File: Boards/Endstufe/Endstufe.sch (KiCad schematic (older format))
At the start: 55 parts, among them J1 HV In, J2 Relais, J3 Audio_In, J4 Übertrager, J5 Gegenkopplung, K1 G6E, P4 6V3_AC, P6 6V3_DC, P8 Bias, T1 KT88, T2 KT88, U1 ECC82, U2 ECC83

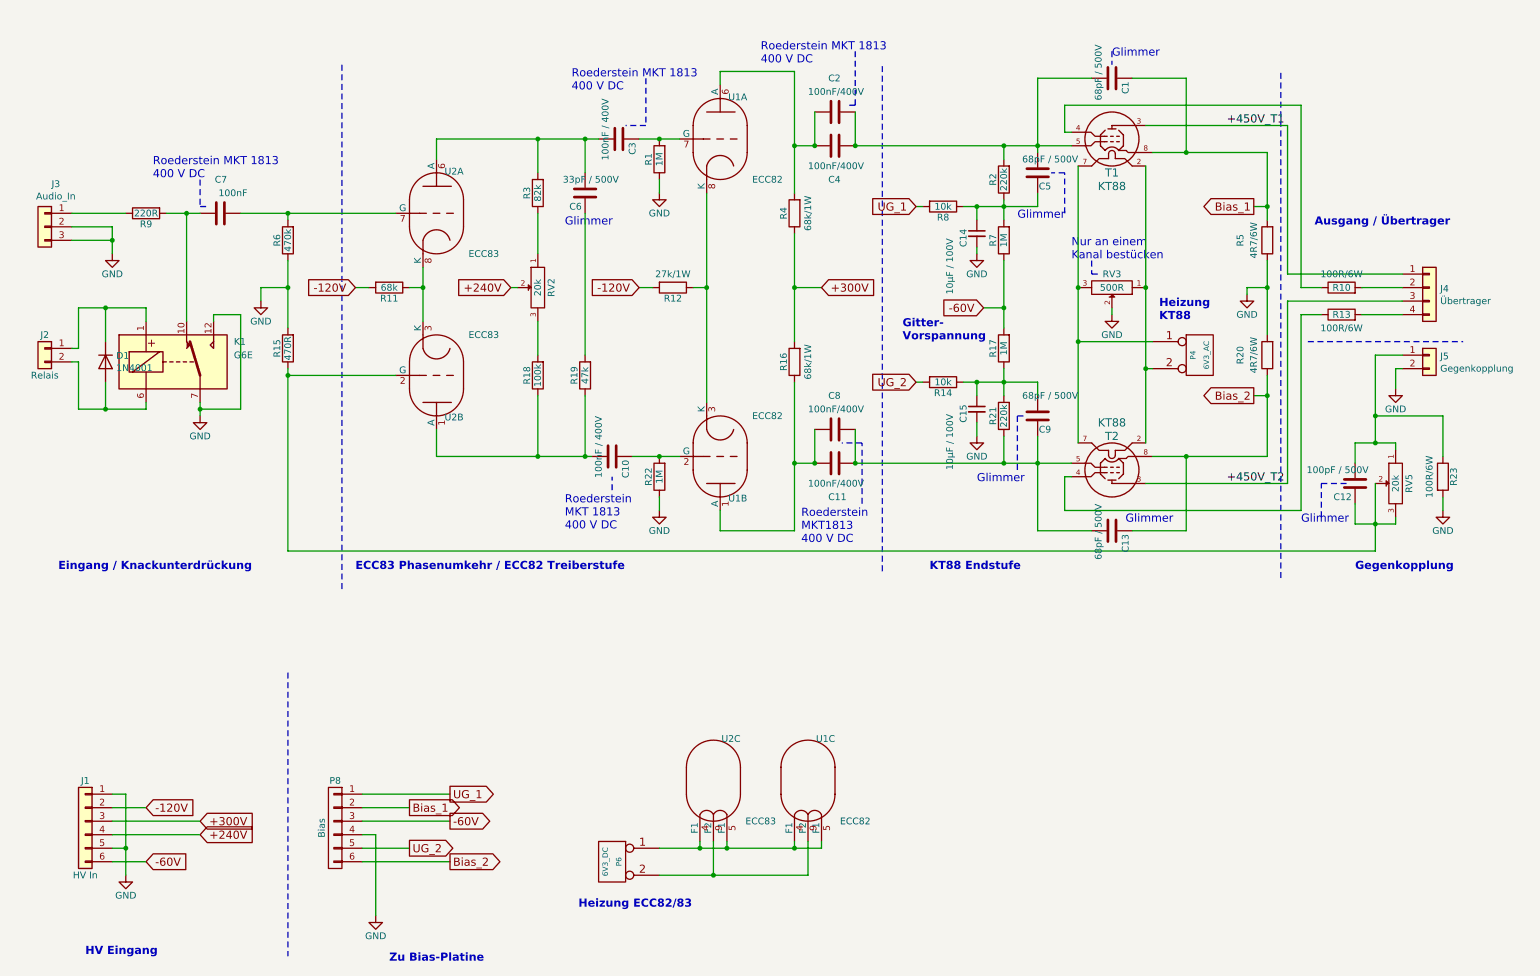
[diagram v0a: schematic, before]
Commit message: Work in progess - many LAyour changes
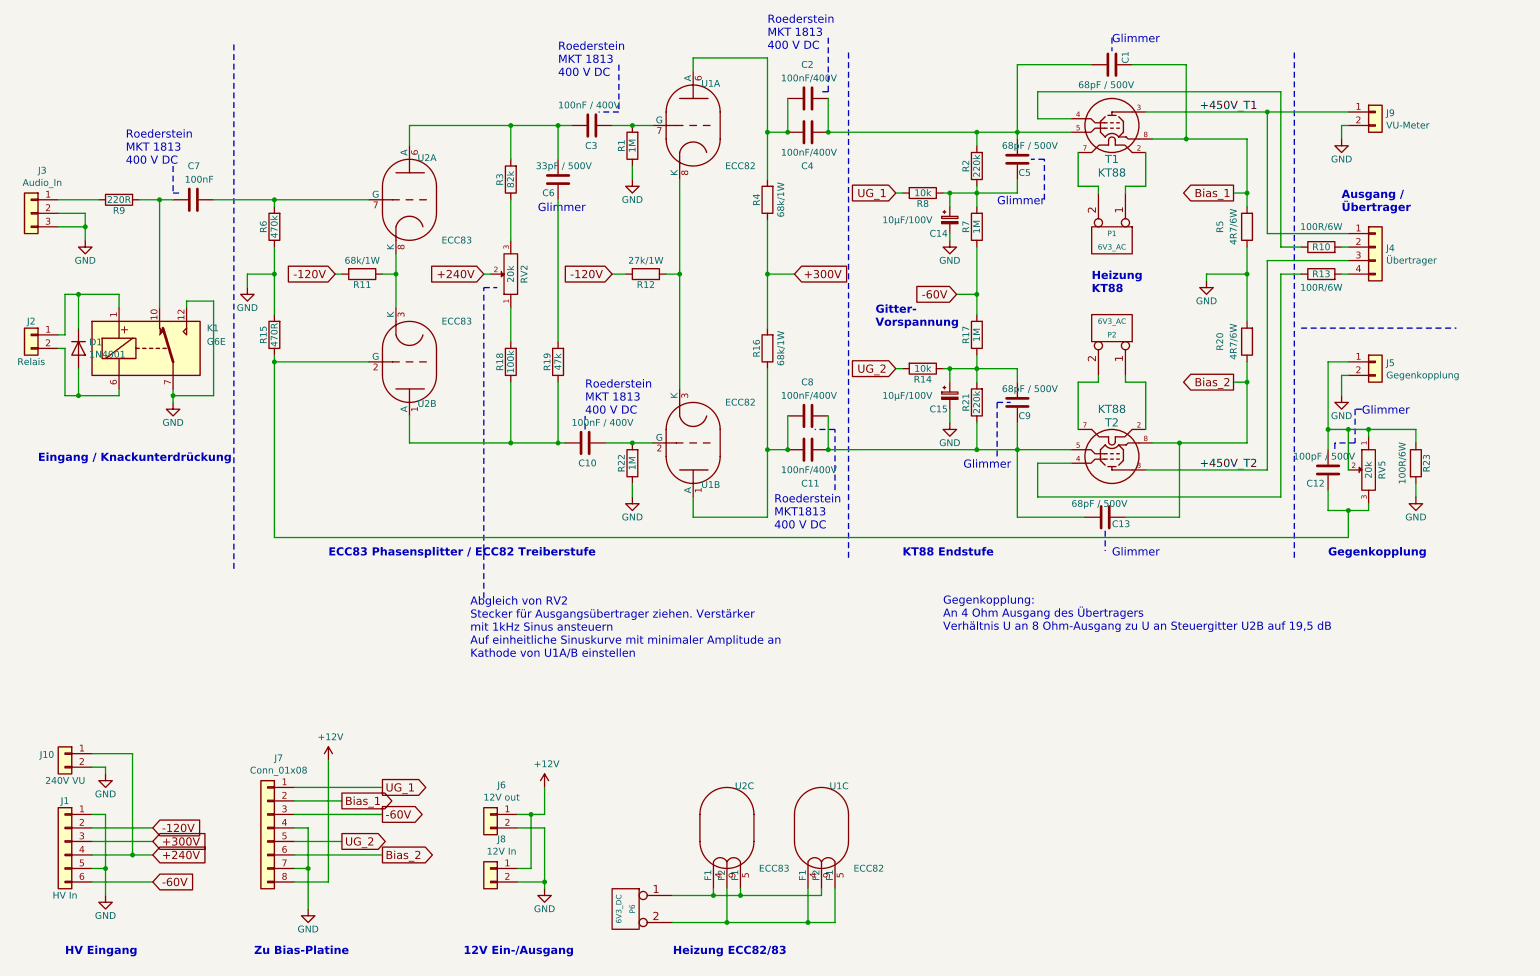
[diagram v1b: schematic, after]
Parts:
- removed C14, C15: 10µF / 100V, Capacitor_THT:C_Radial_D6.3mm_H5.0mm_P2.50mm, symbol Endstufe-rescue:C_Small
- removed P4: 6V3_AC, Connector_TE-Connectivity:TE_MATE-N-LOK_1-770866-x_1x02_P4.14mm_Vertical, symbol Endstufe-rescue:CONN_2
- removed P8: Bias, Connector_PinHeader_2.54mm:PinHeader_2x03_P2.54mm_Vertical, symbol Endstufe-rescue:CONN_01X06
- removed RV3: 500R, Potentiometer_THT:Potentiometer_Piher_PT-10-V10_Vertical, symbol Endstufe-rescue:POT-RESCUE-Endstufe
- added C14, C15: 10µF/100V, Capacitor_THT:CP_Radial_D6.3mm_P2.50mm, symbol Device:CP_Small
- added J10: 240V VU, Connector_TE-Connectivity:TE_MATE-N-LOK_1-770866-x_1x02_P4.14mm_Vertical, symbol Connector_Generic:Conn_01x02
- added J6: 12V out, Connector_Molex:Molex_KK-254_AE-6410-02A_1x02_P2.54mm_Vertical, symbol Connector_Generic:Conn_01x02
- added J7: Conn_01x08, Connector_PinHeader_2.54mm:PinHeader_2x04_P2.54mm_Vertical, symbol Connector_Generic:Conn_01x08
- added J8: 12V In, Connector_Molex:Molex_KK-254_AE-6410-02A_1x02_P2.54mm_Vertical, symbol Connector_Generic:Conn_01x02
- added J9: VU-Meter, Connector_TE-Connectivity:TE_MATE-N-LOK_1-770866-x_1x02_P4.14mm_Vertical, symbol Connector_Generic:Conn_01x02
- added P1, P2: 6V3_AC, Connector_TE-Connectivity:TE_MATE-N-LOK_1-770866-x_1x02_P4.14mm_Vertical, symbol Endstufe-rescue:CONN_2
- C6: footprint Capacitor_THT:C_Disc_D6.0mm_W2.5mm_P5.00mm -> Capacitor_THT:C_Disc_D6.0mm_W4.4mm_P5.00mm
- C7: footprint Capacitor_THT:C_Disc_D3.0mm_W2.0mm_P2.50mm -> Capacitor_THT:C_Axial_L22.0mm_D9.5mm_P27.50mm_Horizontal
- C9: footprint Capacitor_THT:C_Disc_D7.5mm_W2.5mm_P5.00mm -> Capacitor_THT:C_Disc_D7.5mm_W4.4mm_P5.00mm
- R10, R13, R20, R23, R5: footprint Resistor_THT:R_Axial_Power_L25.0mm_W9.0mm_P30.48mm -> Resistor_THT:R_Axial_DIN0922_L20.0mm_D9.0mm_P25.40mm_Horizontal
- R11: value 68k -> 68k/1W; footprint Resistor_THT:R_Axial_DIN0207_L6.3mm_D2.5mm_P10.16mm_Horizontal -> Resistor_THT:R_Axial_DIN0207_L6.3mm_D2.5mm_P15.24mm_Horizontal
- R12: footprint Resistor_THT:R_Axial_DIN0414_L11.9mm_D4.5mm_P20.32mm_Horizontal -> Resistor_THT:R_Axial_DIN0207_L6.3mm_D2.5mm_P15.24mm_Horizontal
- R16, R4: footprint Resistor_THT:R_Axial_DIN0414_L11.9mm_D4.5mm_P15.24mm_Horizontal -> Resistor_THT:R_Axial_DIN0207_L6.3mm_D2.5mm_P10.16mm_Horizontal
- RV2, RV5: footprint Potentiometer_THT:Potentiometer_Piher_PT-10-V10_Vertical -> Potentiometer_THT:Potentiometer_Piher_PT-10-V10_Vertical_Hole
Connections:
- net +240V: now also J10.1 (Pin_1)
- net +450V_T1: now also J9.1 (Pin_1)
- net -60V: now also J7.3 (Pin_3)
- net Bias_1: now also J7.2 (Pin_2)
- net Bias_2: now also J7.6 (Pin_6)
- net GND: now also C14.2, C15.2, J10.2 (Pin_2), J6.2 (Pin_2), J7.4 (Pin_4), J7.7 (Pin_7), J8.2 (Pin_2), J9.2 (Pin_2)
- net UG_1: now also J7.1 (Pin_1)
- net UG_2: now also J7.5 (Pin_5)
- net at T1.2 (f): now also P1.1 (P1); no longer T2.2 (f)
- net at T1.7 (f): now also P1.2 (P2); no longer T2.7 (f)
- net at C12.1, R15.1, RV5.3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: no longer RV5.2
- net at P6.1 (P1), U2.4 (F1), U2.5 (F1): now also U1.9 (F2); no longer U1.4 (F1), U1.5 (F1)
- net at P6.2 (P2), U2.9 (F2): now also U1.4 (F1), U1.5 (F1); no longer U1.9 (F2)
- net at RV2.1: now also R18.2; no longer R3.1
- net at RV2.3: now also R3.1; no longer R18.2
- net at C5.1, R2.1, R7.2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: now also C14.1
- net at C9.2, R14.1, R17.1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: now also C15.1
- net at C12.2, J5.1 (Pin_1), R23.1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: now also RV5.2
- new net: P2.1 (P1), T2.2 (f)
- new net: P2.2 (P2), T2.7 (f)
- new net +12V: J6.1 (Pin_1), J7.8 (Pin_8), J8.1 (Pin_1)
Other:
- note added: "12V Ein-/Ausgang"
- note added: "Abgleich von RV2\nStecker für Ausgangsübertrager ziehen. Verstärker\nmit 1kHz Sinus ansteuern\nAuf einheitliche Sinuskurve mit minimaler Amplitude an\nKathode von U1A/B einstellen"
- note added: "Ausgang / \nÜbertrager"
- note added: "ECC83 Phasensplitter / ECC82 Treiberstufe"
- note added: "Gegenkopplung:\nAn 4 Ohm Ausgang des Übertragers\nVerhältnis U an 8 Ohm-Ausgang zu U an Steuergitter U2B auf 19,5 dB"
- note added: "Roederstein\nMKT 1813\n400 V DC"
- note removed: "Ausgang / Übertrager"
- note removed: "ECC83 Phasenumkehr / ECC82 Treiberstufe"
- note removed: "Nur an einem \nKanal bestücken"
- note removed: "Roederstein MKT 1813\n400 V DC"
- moved on the sheet: C1, C10, C11, C12, C13, C2, C3, C4, C5, C6, C7, C8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
